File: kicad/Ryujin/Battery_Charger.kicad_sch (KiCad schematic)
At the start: 28 parts, among them Q3 BSC014N04LS, Q4 BSC014N04LSI, U6 BQ24650

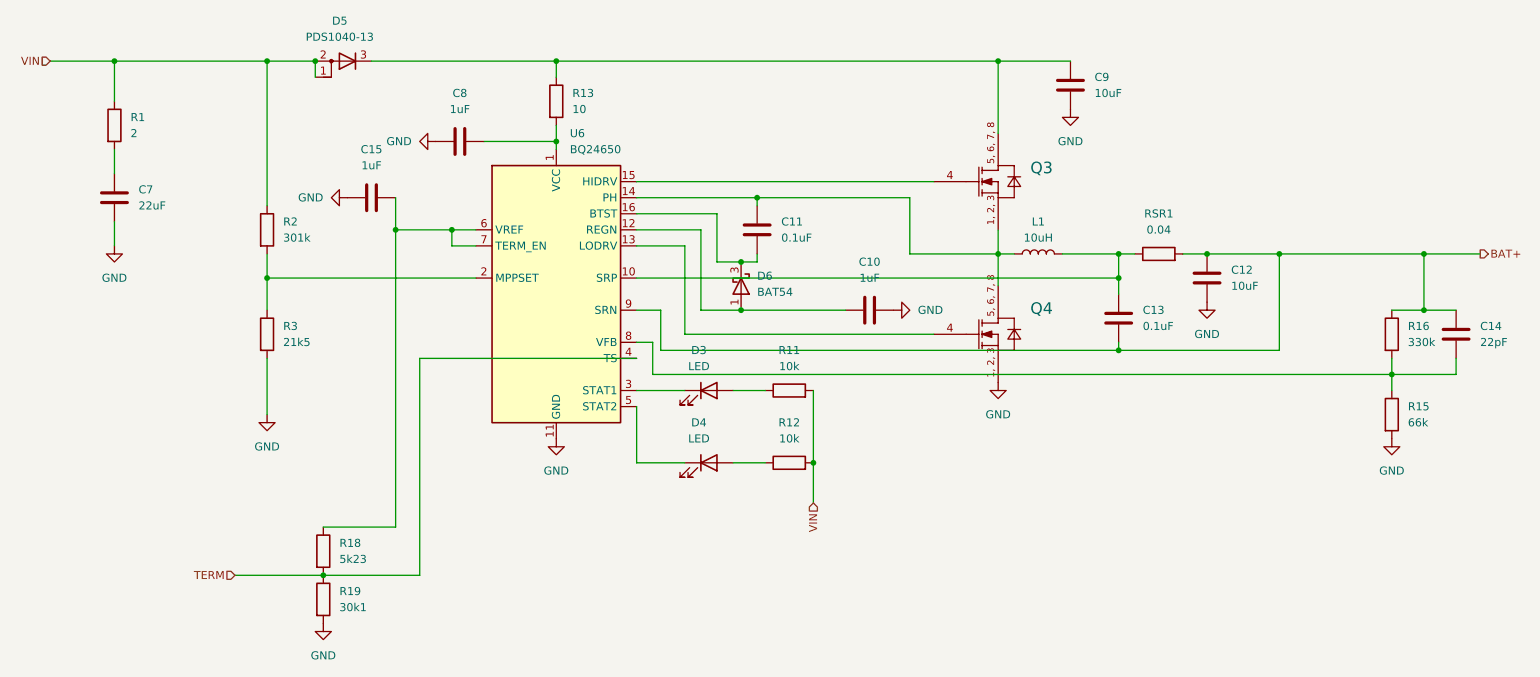
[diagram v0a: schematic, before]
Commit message: Ulysses
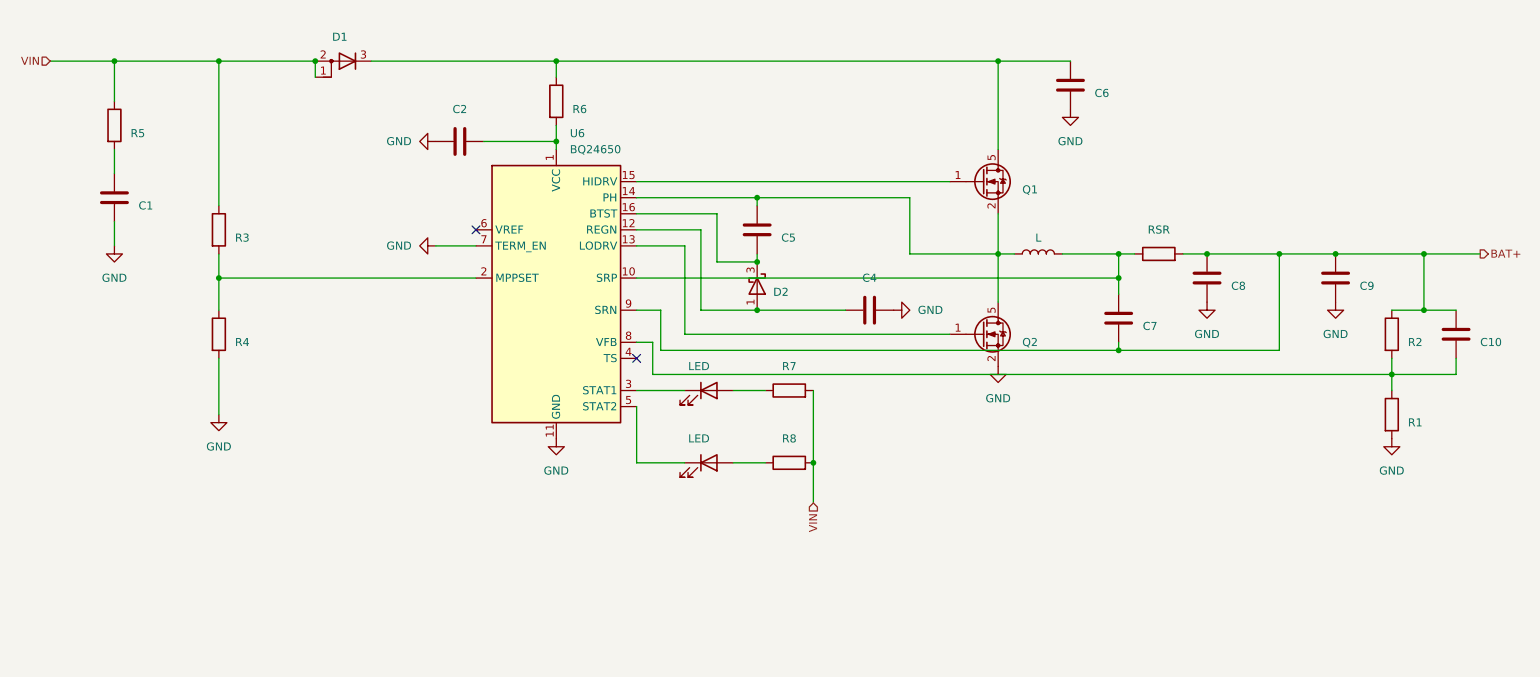
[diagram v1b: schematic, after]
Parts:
- removed C15: 1uF, Capacitor_SMD:C_0805_2012Metric, symbol Device:C
- removed Q3: BSC014N04LS, footprints:INF-PG-TDSON-8-FL, symbol Infineon:BSC014N04LS
- removed Q4: BSC014N04LSI, footprints:INF-PG-TDSON-8-FL, symbol Infineon:BSC014N04LSI
- removed R18: 5k23, Resistor_SMD:R_0603_1608Metric, symbol Device:R
- removed R19: 30k1, Resistor_SMD:R_0603_1608Metric, symbol Device:R
- added C16: C9, Capacitor_SMD:C_1210_3225Metric, symbol Device:C
- added Q3: Q1, Package_TO_SOT_SMD:LFPAK88, symbol Transistor_FET:SQJQ100E
- added Q4: Q2, Package_TO_SOT_SMD:LFPAK88, symbol Transistor_FET:SQJQ100E
- C10: value 1uF -> C4; MPN 1uF 10% 35V X7R 0805 -> 1uF 35V 0805
- C11: value 0.1uF -> C5; MPN 0.1uF 10% 35V X7R 0805 -> 0.1uF 35V 0805
- C12: value 10uF -> C8; MPN 10uF 20% 35V X7R 1210 -> 10uF 35V 1210
- C13: value 0.1uF -> C7; MPN 0.1uF 10% 35V X7R 0805 -> 0.1uF 35V 0805
- C14: value 22pF -> C10; MPN 22pF 10% 35V X7R 0603 -> 22pF 35V 0603
- C7: value 22uF -> C1; MPN 22uF 10% 35V X7R 1210 -> 2.2uF 35V 1210
- C8: value 1uF -> C2; MPN 1uF 10% 35V X7R 0805 -> 1uF 35V 0805
- C9: value 10uF -> C6; MPN 10uF 20% 35V X7R 1210 -> 10uF 35V 1210
- D5: value PDS1040-13 -> D1
- D6: value BAT54 -> D2
- L1: value 10uH -> L
- R1: value 2 -> R5; footprint Resistor_SMD:R_0603_1608Metric -> Resistor_SMD:R_0805_2012Metric; MPN 2 0603 5% 1W -> 2 0805
- R11: value 10k -> R7; footprint Resistor_SMD:R_0603_1608Metric -> Resistor_SMD:R_0402_1005Metric; MPN 10k 0603 5% 0.1W -> 10k 0402
- R12: value 10k -> R8; footprint Resistor_SMD:R_0603_1608Metric -> Resistor_SMD:R_0402_1005Metric; MPN 10k 0603 5% 0.1W -> 10k 0402
- R13: value 10 -> R6; MPN 10 1206 5% 0.25W -> 10 1206
- R15: value 66k -> R1; footprint Resistor_SMD:R_0603_1608Metric -> Resistor_SMD:R_0402_1005Metric; MPN 66k 0603 0.5% 0.1W -> 100k 0402
- R16: value 330k -> R2; footprint Resistor_SMD:R_0603_1608Metric -> Resistor_SMD:R_0402_1005Metric; MPN 330k 0603 0.5% 0.1W -> 499k 0402
- R2: value 301k -> R3; footprint Resistor_SMD:R_0603_1608Metric -> Resistor_SMD:R_0402_1005Metric; MPN 301k 0603 0.5% 0.1W -> 499k 0402
- R3: value 21k5 -> R4; footprint Resistor_SMD:R_0603_1608Metric -> Resistor_SMD:R_0402_1005Metric; MPN 21.5k 0603 0.5% 0.1W -> 36k 0402
- RSR1: value 0.04 -> RSR
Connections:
- net BAT+: now also C16.1
- net GND: now also U6.7 (TERM_EN), C16.2, Q4.2 (S), Q4.3 (S), Q4.4 (S)
- net at C11.2, L1.1, U6.14 (PH): now also Q3.2 (S), Q3.3 (S), Q3.4 (S), Q4.5 (D)
- net at U6.6 (VREF): no longer U6.7 (TERM_EN)
- net at C9.1, D5.3 (K), R13.1: now also Q3.5 (D)
- net at U6.15 (HIDRV): now also Q3.1 (G)
- net at U6.13 (LODRV): now also Q4.1 (G)
- net TERM: no longer names the net of U6.4 (TS)
- no-connect marks 0 -> 2
